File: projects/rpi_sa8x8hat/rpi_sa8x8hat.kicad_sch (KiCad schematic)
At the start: 5 parts, among them J1 RPi_GPIO

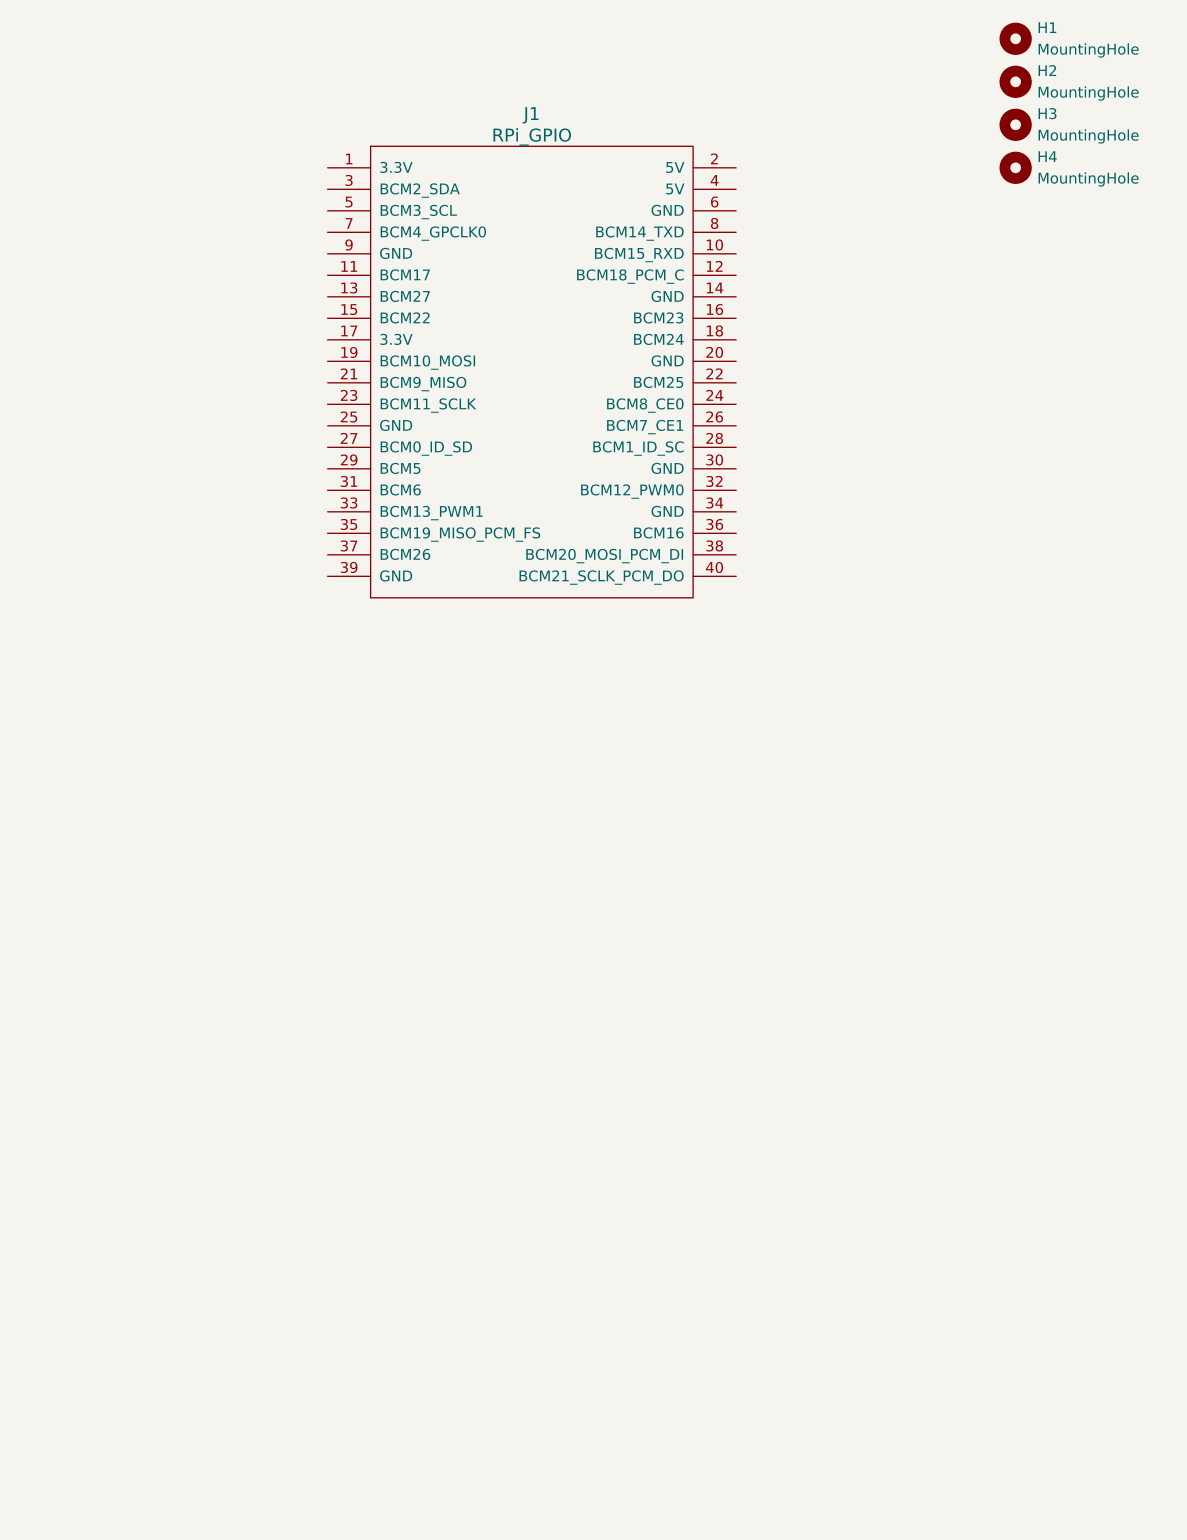
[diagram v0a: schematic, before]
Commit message: .
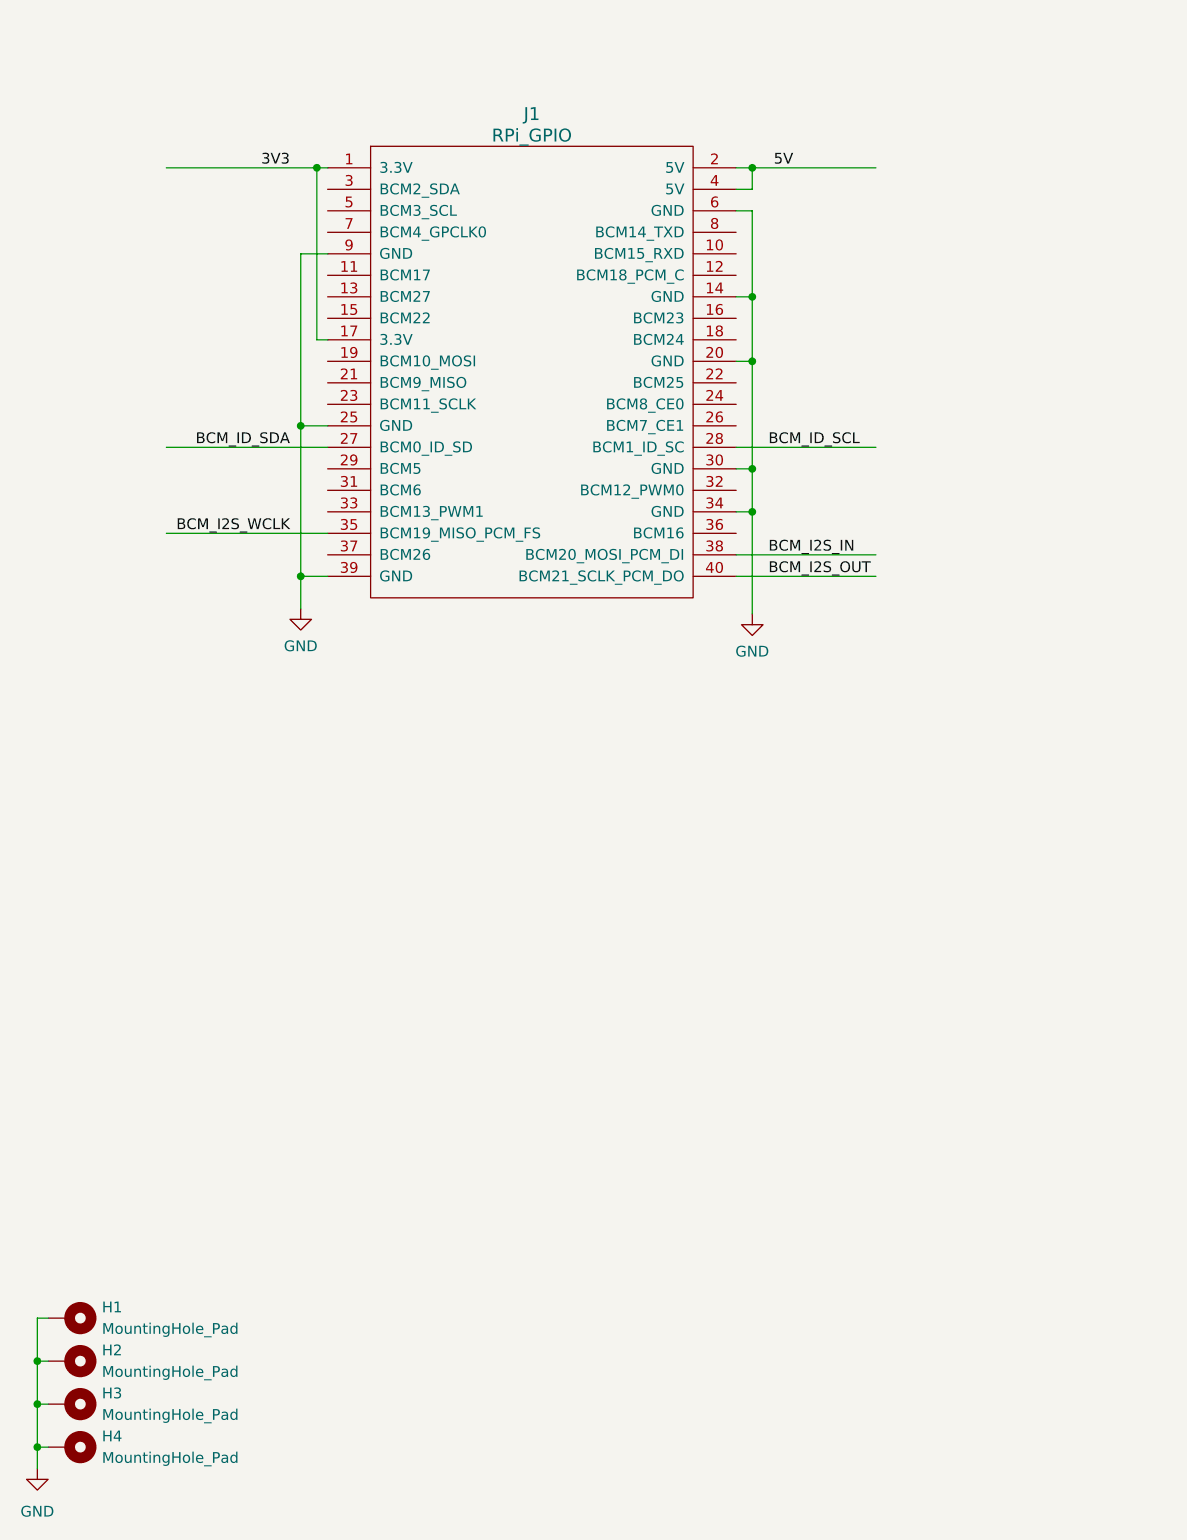
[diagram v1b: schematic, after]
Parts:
- removed H1, H2, H3, H4: MountingHole, RPi_Hat:RPi_Hat_Mounting_Hole, symbol Mechanical:MountingHole
- added H1, H2, H3, H4: MountingHole_Pad, rpi_sa8x8hat:RPi_Hat_Mounting_Hole, symbol Mechanical:MountingHole_Pad
- J1: footprint RPi_Hat:Samtec_HLE-120-02-XXX-DV-BE-XX-XX -> rpi_sa8x8hat:Samtec_HLE-120-02-XXX-DV-BE-XX-XX; symbol RPi_Hat:RPi_GPIO -> rpi_sa8x8hat:RPi_GPIO
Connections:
- net 3V3: now reaches J1.1 (3.3V)
- net 3V3: now also J1.17 (3.3V)
- net GND: now reaches J1.14 (GND)
- net GND: now also J1.20 (GND), J1.25 (GND), J1.30 (GND), J1.34 (GND), J1.39 (GND), J1.6 (GND), J1.9 (GND), H1.1, H2.1, H3.1, H4.1
- net 5V: now reaches J1.2 (5V)
- net 5V: now also J1.4 (5V)
- net BCM_ID_SDA: now reaches J1.27 (BCM0_ID_SD)
- net BCM_ID_SCL: now reaches J1.28 (BCM1_ID_SC)
- net BCM_I2S_WCLK: now reaches J1.35 (BCM19_MISO_PCM_FS)
- net BCM_I2S_IN: now reaches J1.38 (BCM20_MOSI_PCM_DI)
- net BCM_I2S_OUT: now reaches J1.40 (BCM21_SCLK_PCM_DO)
